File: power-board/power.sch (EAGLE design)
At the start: 2 parts, among them IC1 7805TV

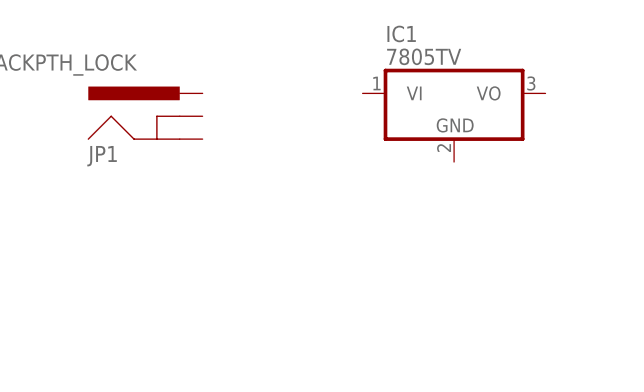
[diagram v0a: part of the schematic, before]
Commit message: pow
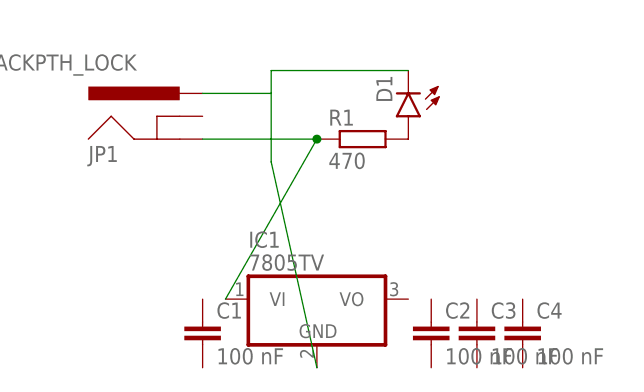
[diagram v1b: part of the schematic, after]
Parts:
- added C1, C2, C3, C4: 100 nF, resistor:C-EU025-025X050
- added D1: (no value), SparkFun-LED:LED5MM
- added R1: 470, resistor:R-EU_0207/10
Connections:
- new net N$1: IC1.VI, JP1.GND, R1.1
- new net N$2: D1.C, IC1.GND, JP1.PWR
- new net N$3: D1.A, R1.2
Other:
- moved on the sheet: IC1
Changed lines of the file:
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@@
 <part name="JP1" library="SparkFun-Connectors" deviceset="POWER_JACK" device="PTH_LOCK"/>
 <part name="IC1" library="linear" deviceset="78*" device="TV" technology="05"/>
+<part name="D1" library="SparkFun-LED" deviceset="LED" device="5MM"/>
+<part name="R1" library="resistor" deviceset="R-EU_" device="0207/10" value="470"/>
+<part name="C1" library="resistor" deviceset="C-EU" device="025-025X050" value="100 nF"/>
+<part name="C2" library="resistor" deviceset="C-EU" device="025-025X050" value="100 nF"/>
+<part name="C3" library="resistor" deviceset="C-EU" device="025-025X050" value="100 nF"/>
+<part name="C4" library="resistor" deviceset="C-EU" device="025-025X050" value="100 nF"/>
 </parts>
 <sheets>
@@
 <attribute name="NAME" x="38.1" y="60.96" size="1.778" layer="95"/>
 </instance>
-<instance part="IC1" gate="A1" x="78.74" y="68.58"/>
+<instance part="IC1" gate="A1" x="63.5" y="45.72"/>
+<instance part="D1" gate="G$1" x="73.66" y="66.04" rot="R180"/>
+<instance part="R1" gate="G$1" x="68.58" y="63.5"/>
+<instance part="C1" gate="G$1" x="50.8" y="43.18"/>
+<instance part="C2" gate="G$1" x="76.2" y="43.18"/>
+<instance part="C3" gate="G$1" x="81.28" y="43.18"/>
+<instance part="C4" gate="G$1" x="86.36" y="43.18"/>
 </instances>
 <busses>
 </busses>
 <nets>
+<net name="N$1" class="0">
+<segment>
+<pinref part="JP1" gate="G$1" pin="GND"/>
+<pinref part="IC1" gate="A1" pin="VI"/>
+<wire x1="50.8" y1="63.5" x2="63.5" y2="63.5" width="0.1524" layer="91"/>
+<wire x1="63.5" y1="63.5" x2="53.34" y2="45.72" width="0.1524" layer="91"/>
+<pinref part="R1" gate="G$1" pin="1"/>
+<junction x="63.5" y="63.5"/>
+</segment>
+</net>
+<net name="N$2" class="0">
+<segment>
+<pinref part="JP1" gate="G$1" pin="PWR"/>
+<wire x1="50.8" y1="68.58" x2="58.42" y2="68.58" width="0.1524" layer="91"/>
+<wire x1="58.42" y1="68.58" x2="58.42" y2="60.96" width="0.1524" layer="91"/>
+<pinref part="IC1" gate="A1" pin="GND"/>
+<wire x1="58.42" y1="60.96" x2="63.5" y2="38.1" width="0.1524" layer="91"/>
+<pinref part="D1" gate="G$1" pin="C"/>
+<wire x1="73.66" y1="71.12" x2="58.42" y2="71.12" width="0.1524" layer="91"/>
+<wire x1="58.42" y1="71.12" x2="58.42" y2="68.58" width="0.1524" layer="91"/>
+</segment>
+</net>
+<net name="N$3" class="0">
+<segment>
+<pinref part="R1" gate="G$1" pin="2"/>
+<pinref part="D1" gate="G$1" pin="A"/>
+</segment>
+</net>
 </nets>
 </sheet>

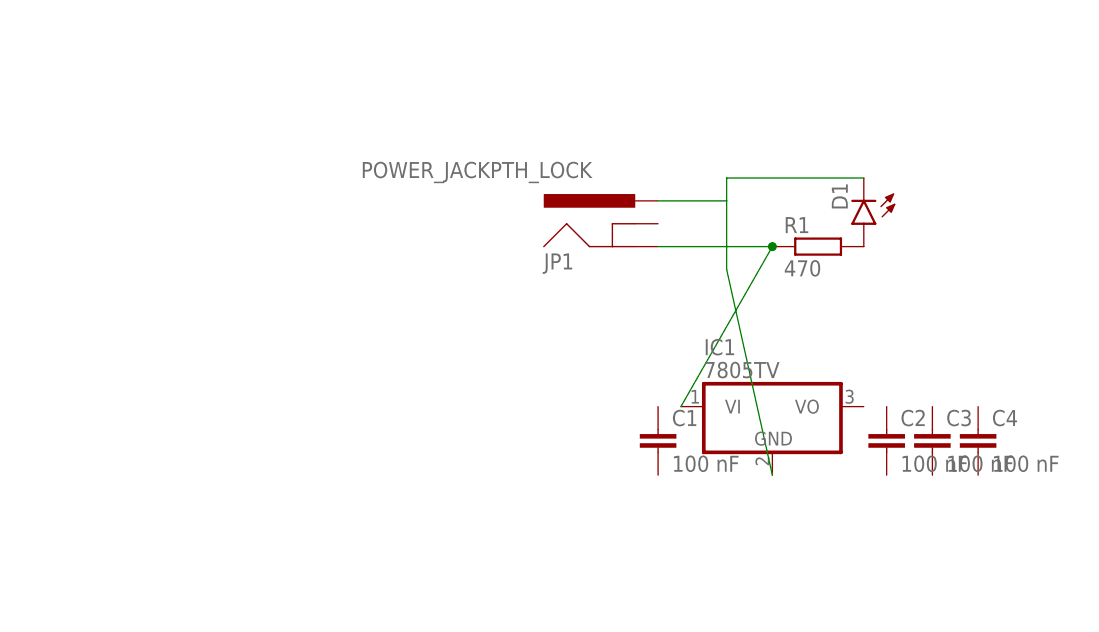
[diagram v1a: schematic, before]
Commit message: power board ok
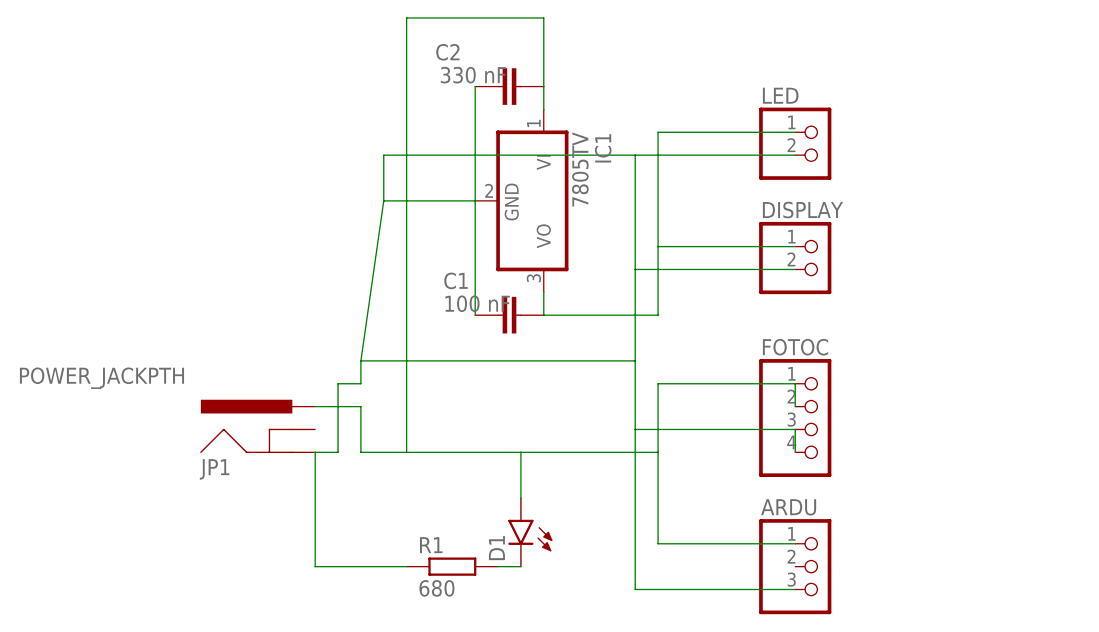
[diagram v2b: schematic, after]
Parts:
- removed C3, C4: 100 nF, resistor:C-EU025-025X050
- added ARDU: (no value), pinhead:PINHD-1X3
- added DISPLAY, LED: (no value), pinhead:PINHD-1X2
- added FOTOC: (no value), pinhead:PINHD-1X4
- C2: value 100 nF -> 330 nF
- JP1: value POWER_JACKPTH_LOCK -> POWER_JACKPTH; device SparkFun-Connectors:POWER_JACKPTH_LOCK -> SparkFun-Connectors:POWER_JACKPTH
- R1: value 470 -> 680
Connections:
- removed net N$3: D1.A, R1.2
- new net N$5: ARDU.3, C1.2, C2.1, DISPLAY.2, FOTOC.3, FOTOC.4, IC1.GND, JP1.GND, LED.2, R1.1
- new net N$6: C1.1, DISPLAY.1, IC1.VO, LED.1
- net N$1: now also D1.C, R1.2; no longer IC1.VI, JP1.GND, R1.1
- net N$2: now also ARDU.1, C2.2, D1.A, FOTOC.1, FOTOC.2, IC1.VI; no longer D1.C, IC1.GND
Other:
- moved on the sheet: C1, C2, D1, IC1, JP1, R1
